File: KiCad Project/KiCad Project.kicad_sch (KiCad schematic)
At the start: 42 parts, among them J1 USB_C_Receptacle_USB2.0_16P, J2 XT30PW-M, Q1 CSD23280F3, U1 STM32F103C8T6, U2 ICM-42670-P, U3 BME280, U4 AP63203WU, U5 AZ1117CH2-3.3, U6 ESD122DMXR, U7 TPD1E10B09DPYR, Y1 ECS-2520MV-160-CN-TR

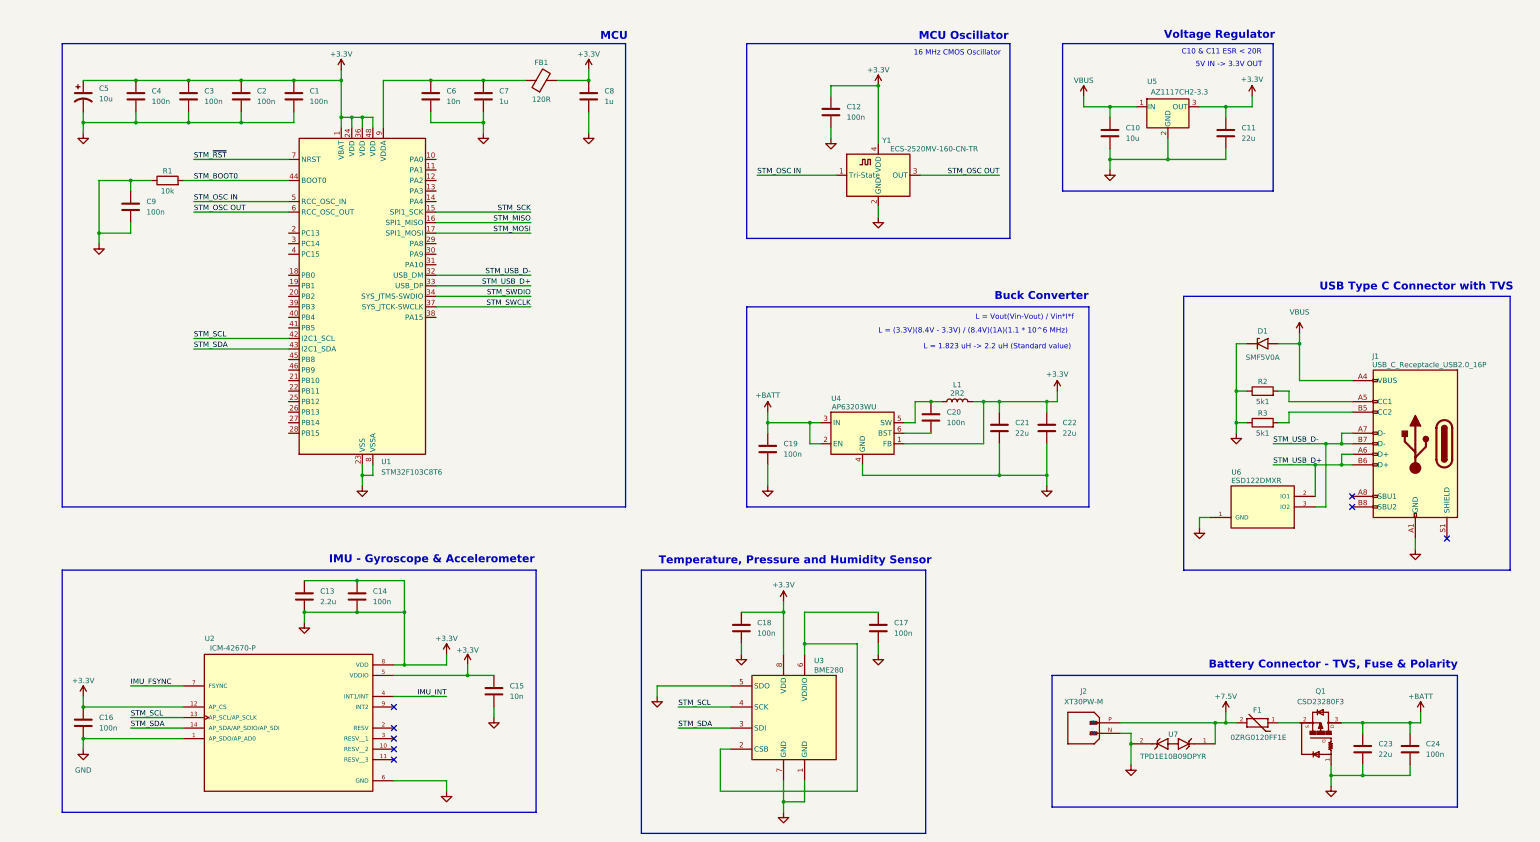
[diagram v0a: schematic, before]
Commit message: 2025/09/12
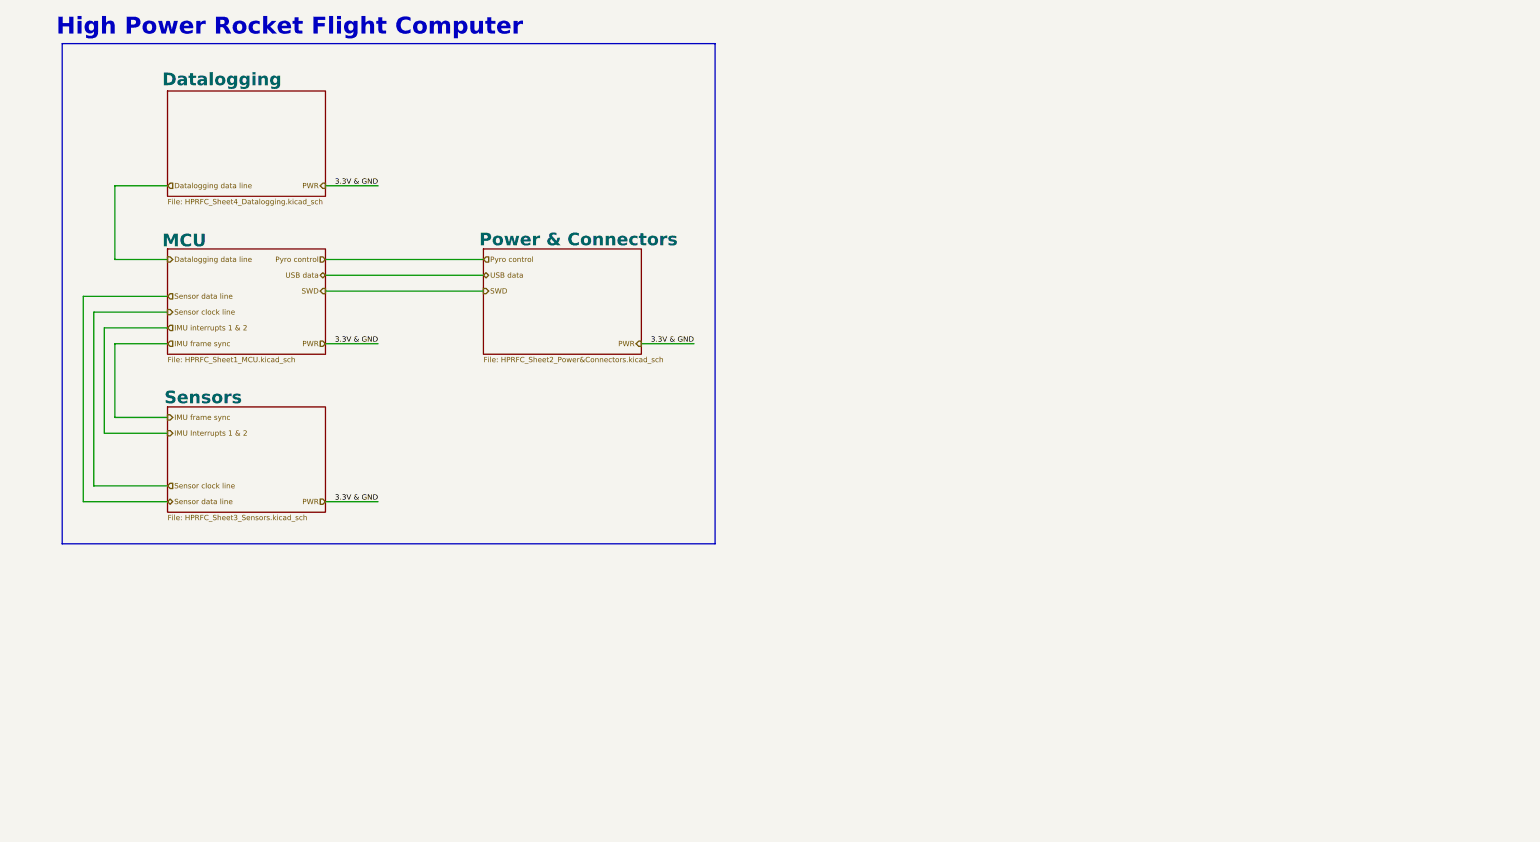
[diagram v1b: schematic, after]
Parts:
- removed C1, C12, C14, C16, C17, C18, C19, C2, C20, C24, C3, C4, C9: 100n, symbol Device:C
- removed C10: 10u, symbol Device:C
- removed C11, C21, C22, C23: 22u, symbol Device:C
- removed C13: 2.2u, symbol Device:C
- removed C15, C6: 10n, symbol Device:C
- removed C5: 10u, symbol Device:C_Polarized_US
- removed C7, C8: 1u, symbol Device:C
- removed D1: SMF5V0A, Diode_SMD:D_SMF, symbol Diode:SMF5V0A
- removed F1: 0ZRG0120FF1E, 0ZRG0120FF1E:FUSRB510W51L690T300H1170, symbol 0ZRG0120FF1E:0ZRG0120FF1E
- removed FB1: 120R, symbol Device:FerriteBead
- removed J1: USB_C_Receptacle_USB2.0_16P, symbol Connector:USB_C_Receptacle_USB2.0_16P
- removed J2: XT30PW-M, XT30PW-M:AMASS_XT30PW-M, symbol XT30PW-M:XT30PW-M
- removed L1: 2R2, symbol Device:L
- removed Q1: CSD23280F3, CSD23280F3:TRANS_CSD23280F3, symbol CSD23280F3:CSD23280F3
- removed R1: 10k, symbol Device:R
- removed R2, R3: 5k1, symbol Device:R
- removed U1: STM32F103C8T6, Package_QFP:LQFP-48_7x7mm_P0.5mm, symbol MCU_ST_STM32F1:STM32F103C8Tx
- removed U2: ICM-42670-P, ICM-42670-P:XDCR_ICM-42670-P, symbol ICM-42670-P:ICM-42670-P
- removed U3: BME280, Package_LGA:Bosch_LGA-8_2.5x2.5mm_P0.65mm_ClockwisePinNumbering, symbol Sensor:BME280
- removed U4: AP63203WU, Package_TO_SOT_SMD:TSOT-23-6, symbol Regulator_Switching:AP63203WU
- removed U5: AZ1117CH2-3.3, Package_TO_SOT_SMD:SOT-223-3_TabPin2, symbol Regulator_Linear:AZ1117CH2-3.3
- removed U6: ESD122DMXR, ESD122DMXR:IC_ESD122DMXR, symbol ESD122DMXR:ESD122DMXR
- removed U7: TPD1E10B09DPYR, TPD1E10B09DPYR:DIO_TPD1E10B09DPYR, symbol TPD1E10B09DPYR:TPD1E10B09DPYR
- removed Y1: ECS-2520MV-160-CN-TR, Oscillator:Oscillator_SMD_ECS_2520MV-xxx-xx-4Pin_2.5x2.0mm, symbol Oscillator:ECS-2520MV-xxx-xx
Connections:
- no-connect marks 8 -> 0
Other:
- added sheet Datalogging (HPRFC_Sheet4_Datalogging.kicad_sch)
- added sheet MCU (HPRFC_Sheet1_MCU.kicad_sch)
- added sheet Power & Connectors (HPRFC_Sheet2_Power&Connectors.kicad_sch)
- added sheet Sensors (HPRFC_Sheet3_Sensors.kicad_sch)
- note added: "High Power Rocket Flight Computer"
- note removed: "16 MHz CMOS Oscillator"
- note removed: "5V IN -> 3.3V OUT"
- note removed: "Battery Connector - TVS, Fuse & Polarity"
- note removed: "Buck Converter"
- note removed: "C10 & C11 ESR < 20R"
- note removed: "IMU - Gyroscope & Accelerometer"
- note removed: "L = (3.3V)(8.4V - 3.3V) / (8.4V)(1A)(1.1 * 10^6 MHz)"
- note removed: "L = 1.823 uH -> 2.2 uH (Standard value)"
- note removed: "L = Vout(Vin-Vout) / Vin*I*f"
- note removed: "MCU"
- note removed: "MCU Oscillator"
- note removed: "Temperature, Pressure and Humidity Sensor"
- note removed: "USB Type C Connector with TVS"
- note removed: "Voltage Regulator"
- company: (none) -> Edward Sicoe
- title: (none) -> High Power Rocket Flight Computer - Hierarchical Page
